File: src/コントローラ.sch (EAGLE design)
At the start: 36 parts

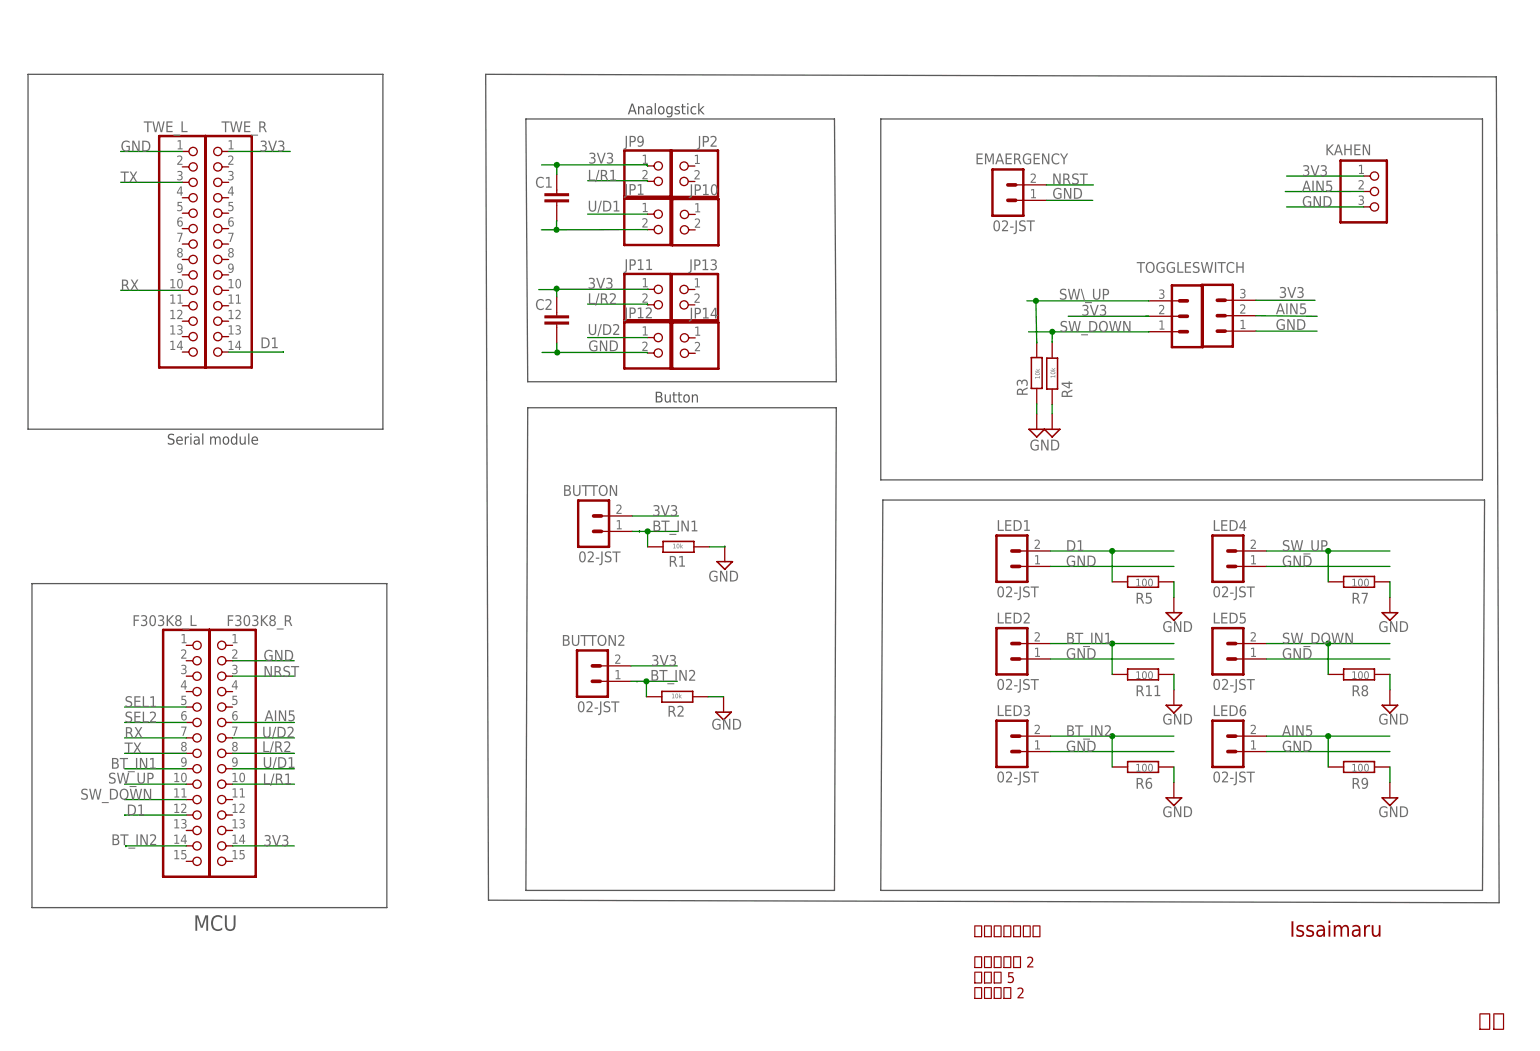
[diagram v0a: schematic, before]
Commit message: [add]コントローラ　Aoi
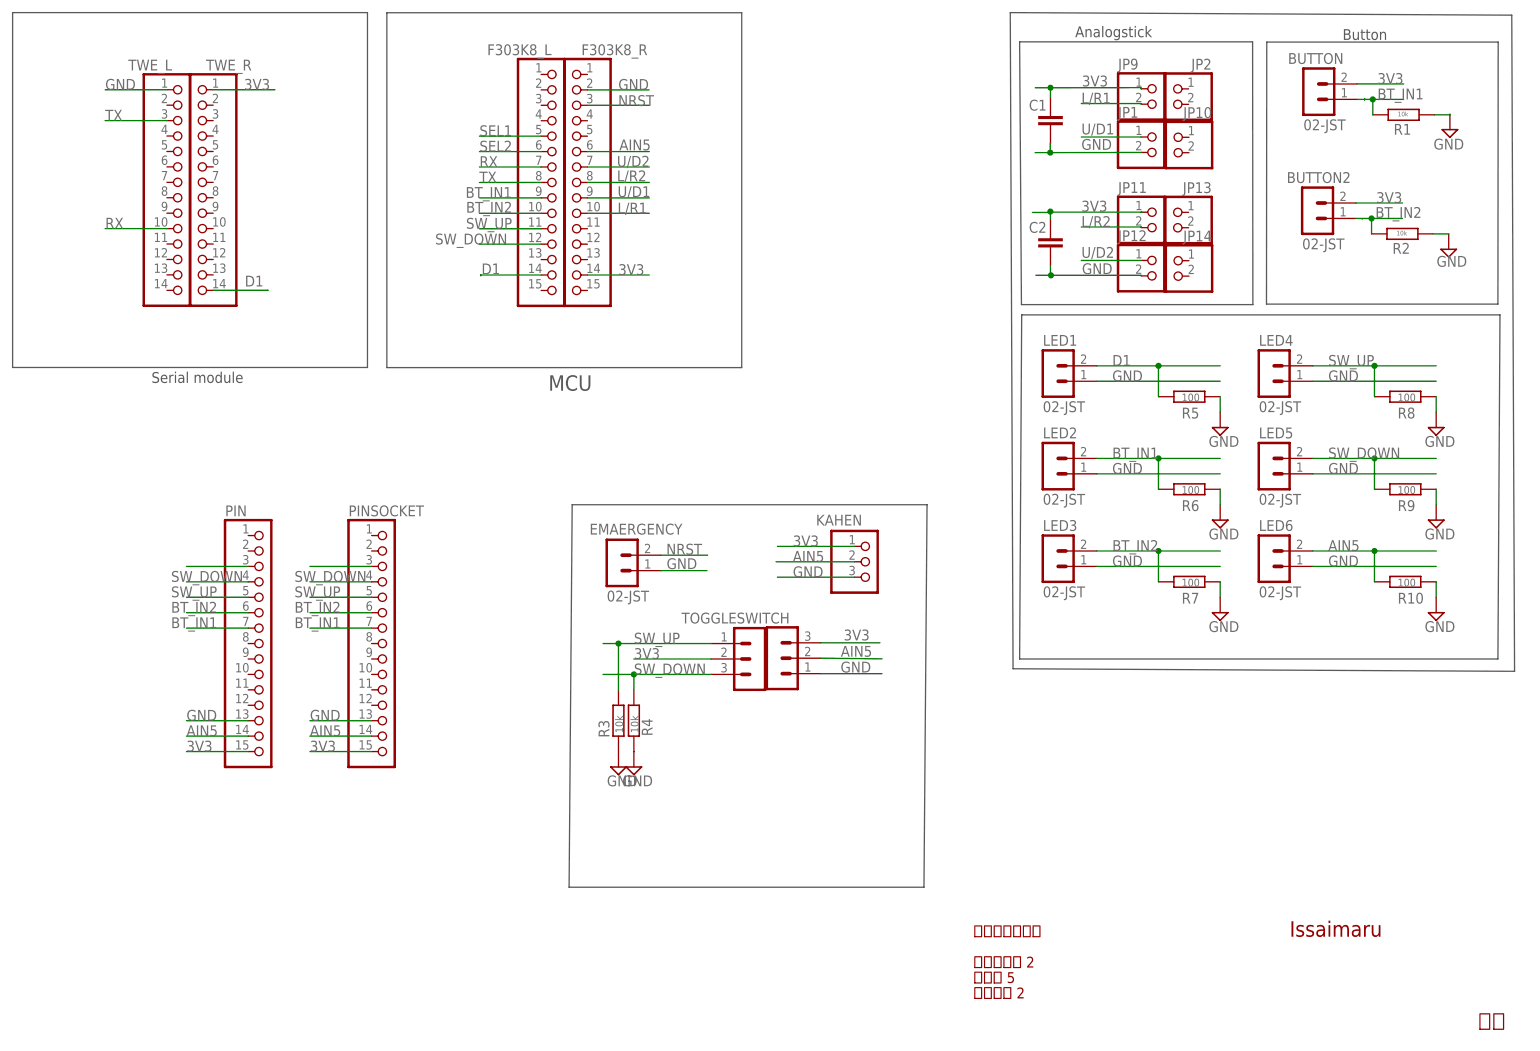
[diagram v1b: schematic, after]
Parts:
- removed R11: 100, rcl:R-EU_0204/7
- removed TOGLLESWITCH: (no value), con-jst-xh (1):03-JST
- added PIN, PINSOCKET: (no value), pinhead:PINHD-1X15
- added R10: 100, rcl:R-EU_0204/7
- added TOGGLESWITCH: (no value), con-jst-xh (1):03-JST
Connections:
- removed net SW\_UP: R3.2, TOGLLESWITCH.3
- new net N$8: PINSOCKET.3
- net 3V3: now also PIN.15, PINSOCKET.15, TOGGLESWITCH.2; no longer TOGLLESWITCH.2
- net AIN5: now also PIN.14, PINSOCKET.14, R10.1; no longer R9.1
- net BT_IN1: now also PIN.7, PINSOCKET.7, R6.1; no longer R11.1
- net BT_IN2: now also F303K8_L.10, PIN.6, PINSOCKET.6, R7.1; no longer F303K8_L.14, R6.1
- net D1: now also F303K8_L.14; no longer F303K8_L.12
- net GND: now also C1.2, JP1.2, PIN.13, PINSOCKET.13, R10.2; no longer R11.2
- net N$1: now also PIN.3; no longer C1.2, JP1.2
- net SW_DOWN: now also F303K8_L.12, PIN.4, PINSOCKET.4, R9.1, TOGGLESWITCH.3; no longer F303K8_L.11, R8.1, TOGLLESWITCH.1
- net SW_UP: now also F303K8_L.11, PIN.5, PINSOCKET.5, R3.2, R8.1, TOGGLESWITCH.1; no longer F303K8_L.10, R7.1
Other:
- note removed: "TOGGLESWITCH"
- moved on the sheet: BUTTON, BUTTON2, C1, C2, EMAERGENCY, F303K8_L, F303K8_R, JP1, JP10, JP11, JP12, JP13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
